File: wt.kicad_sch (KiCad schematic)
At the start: 47 parts, among them U2 STM32F407VGTx

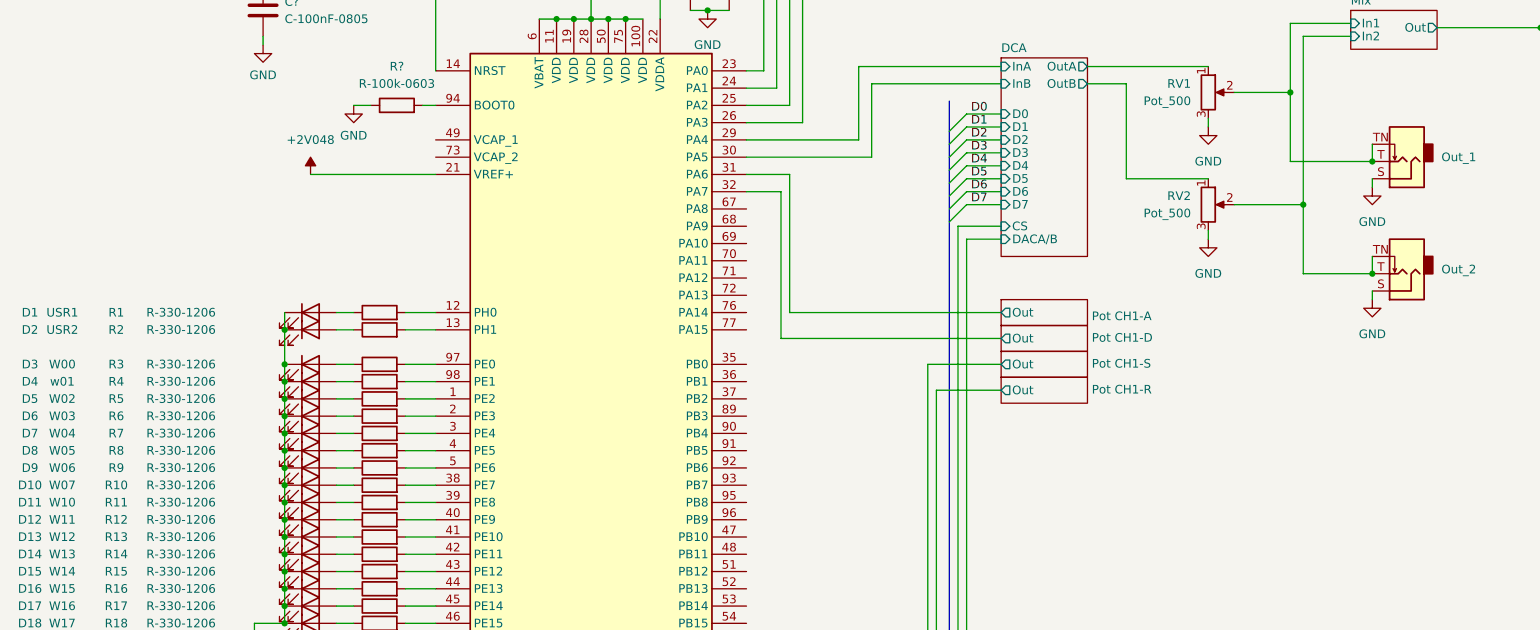
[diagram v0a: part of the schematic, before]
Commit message: WIP
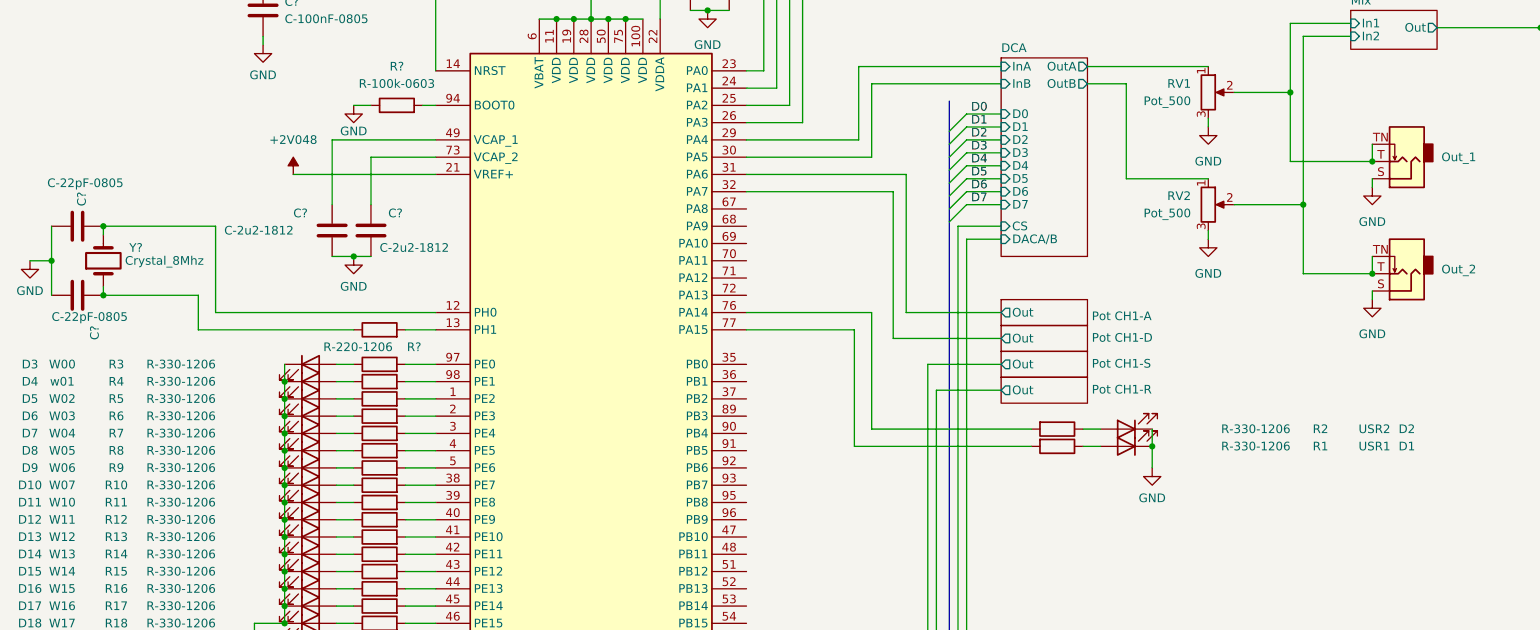
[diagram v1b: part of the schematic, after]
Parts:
- added C? (x2): C-2u2-1812, Capacitor_SMD:C_1812_4532Metric_Pad1.57x3.40mm_HandSolder, symbol eurorack:C-2u2-1812
- added C? (x2): C-22pF-0805, Capacitor_SMD:C_0805_2012Metric_Pad1.18x1.45mm_HandSolder, symbol eurorack:C-22pF-0805
- added R?: R-220-1206, Resistor_SMD:R_1206_3216Metric_Pad1.30x1.75mm_HandSolder, symbol eurorack:R-220-1206
- added Y?: Crystal_8Mhz, eurorack:HC49-4HSMX, symbol eurorack:Crystal_8Mhz
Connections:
- net GND: now also C?.2, C?.2, C?.2, C?.2
- net at R1.2: now also U2.77 (PA15); no longer U2.12 (PH0)
- net at U2.13 (PH1): now also R?.2; no longer R2.2
- net at U2.49 (VCAP_1): now also C?.1
- net at U2.73 (VCAP_2): now also C?.1
- net at U2.76 (PA14): now also R2.2
- new net: C?.1, U2.12 (PH0), Y?.2
- new net: C?.1, R?.1, Y?.1
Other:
- moved on the sheet: D1, D2, R1, R2
